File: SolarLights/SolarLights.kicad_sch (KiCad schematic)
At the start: 25 parts, among them J1 BAT GND, J2 BAT 12V, J3 SWITCH IN, J4 SWITCH 12V, J5 SWITCH GND, J6 PROG, U1 ATtiny1616

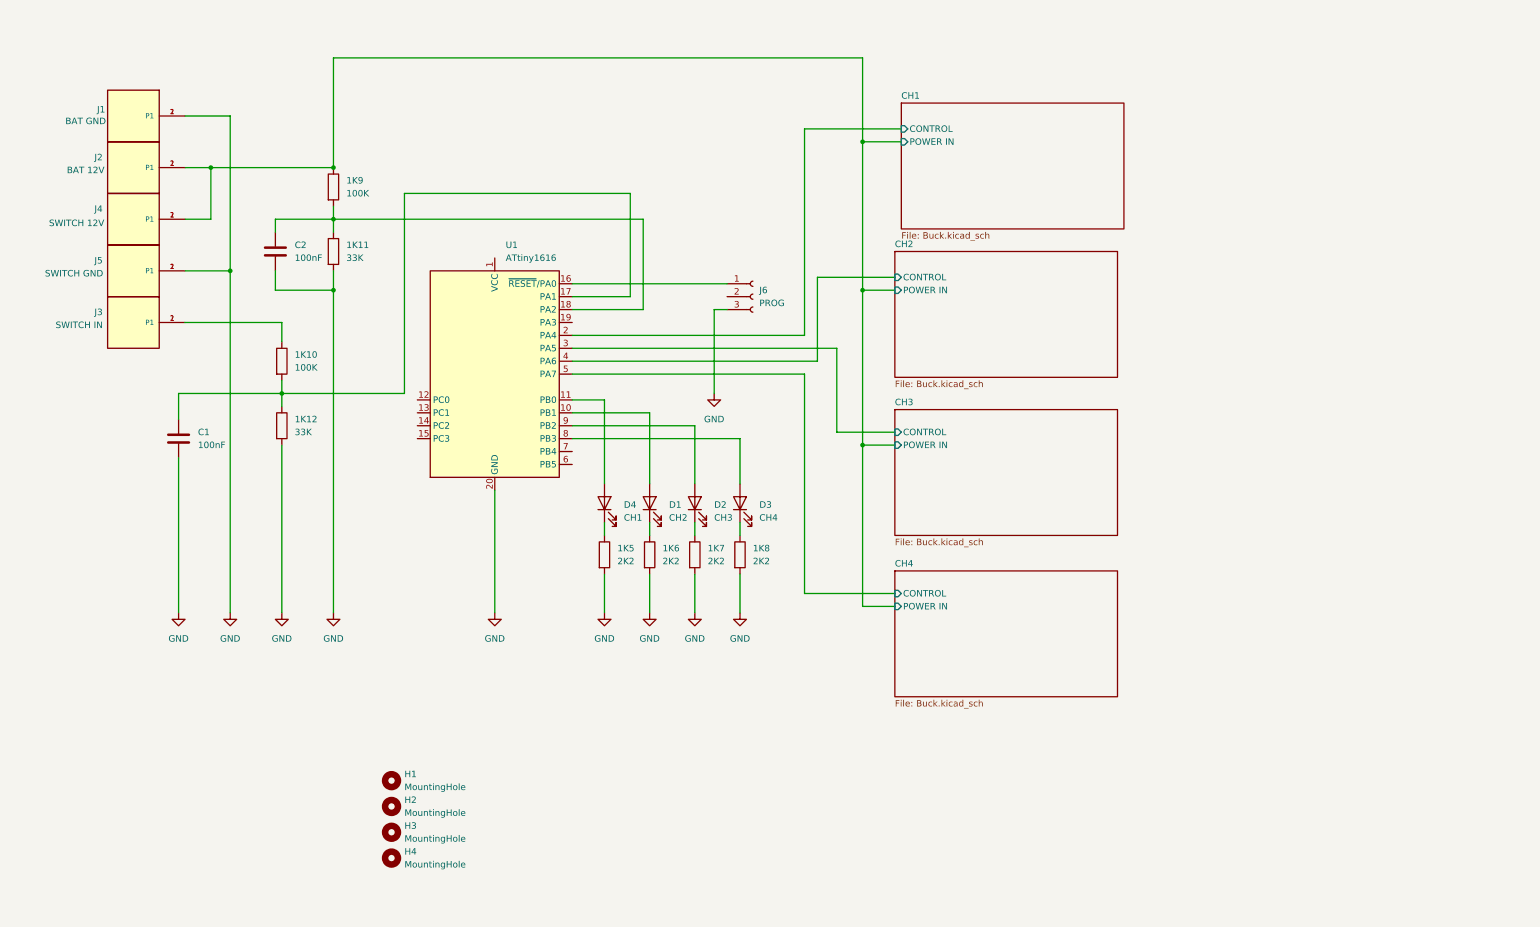
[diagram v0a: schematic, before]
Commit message: solar lights
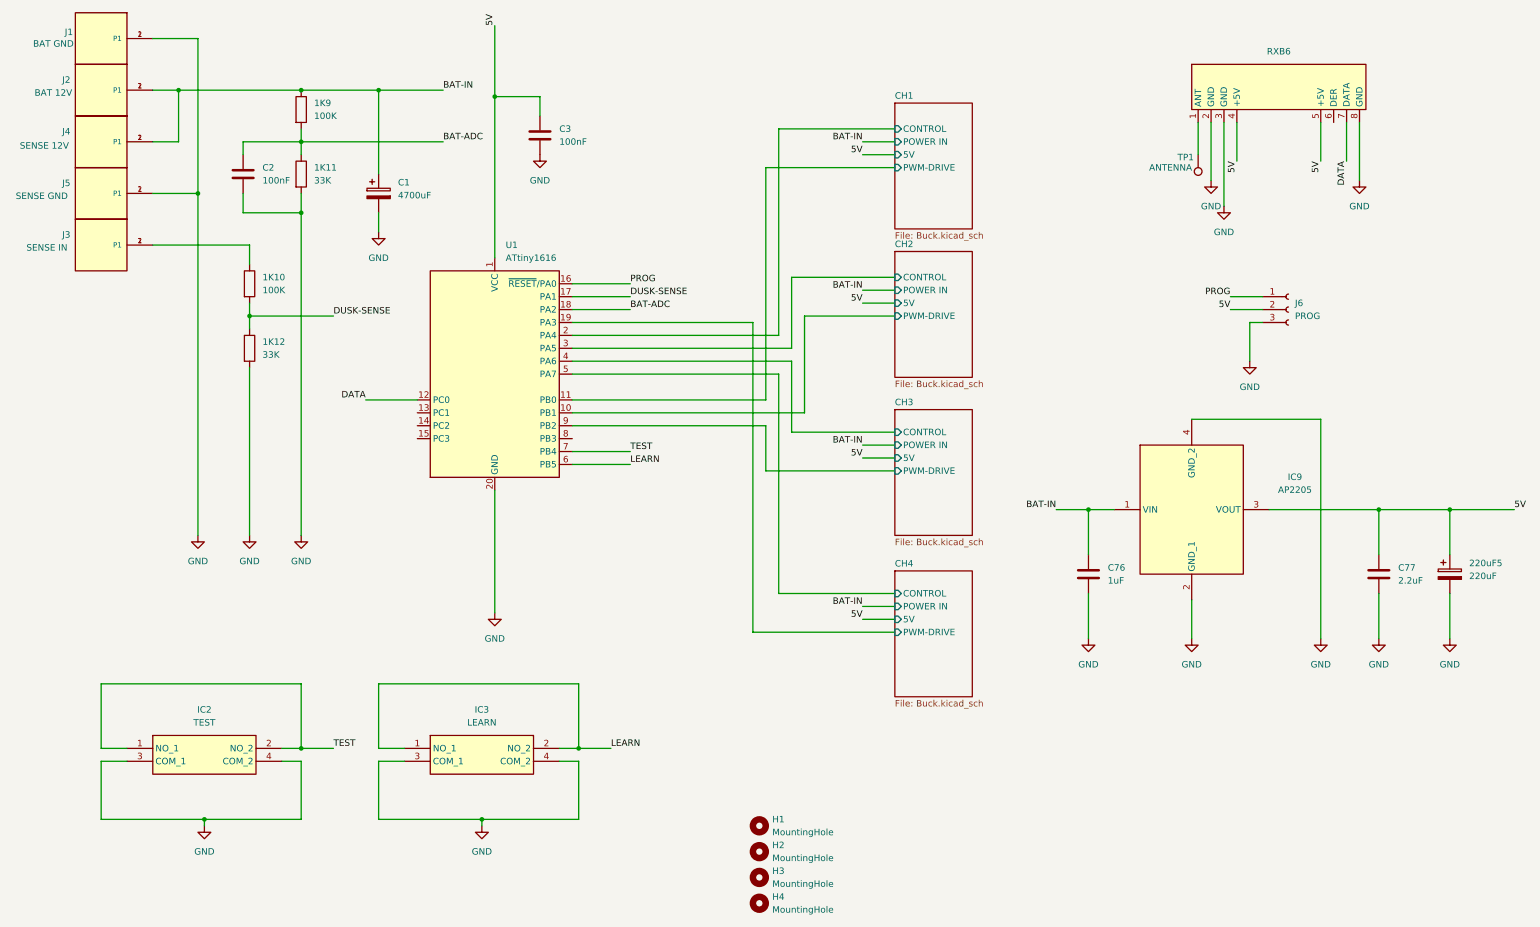
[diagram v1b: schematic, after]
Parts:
- removed 1K5, 1K6, 1K7, 1K8: 2K2, Resistor_SMD:R_0805_2012Metric_Pad1.20x1.40mm_HandSolder, symbol Device:R
- removed C1: 100nF, Capacitor_SMD:C_1206_3216Metric_Pad1.33x1.80mm_HandSolder, symbol Device:C
- removed D1: CH2, LED_THT:LED_D5.0mm, symbol Device:LED
- removed D2: CH3, LED_THT:LED_D5.0mm, symbol Device:LED
- removed D3: CH4, LED_THT:LED_D5.0mm, symbol Device:LED
- removed D4: CH1, LED_THT:LED_D5.0mm, symbol Device:LED
- added 220uF5: 220uF, Capacitor_THT:CP_Radial_D6.3mm_P2.50mm, symbol Device:C_Polarized
- added C1: 4700uF, Capacitor_THT:CP_Radial_D16.0mm_P7.50mm, symbol Device:C_Polarized
- added C3: 100nF, Capacitor_SMD:C_1206_3216Metric_Pad1.33x1.80mm_HandSolder, symbol Device:C
- added C76: 1uF, Capacitor_SMD:C_1206_3216Metric_Pad1.33x1.80mm_HandSolder, symbol Device:C
- added C77: 2.2uF, Capacitor_SMD:C_0805_2012Metric_Pad1.18x1.45mm_HandSolder, symbol Device:C
- added IC2: TEST, Custom:TS026650BK100SCRD, symbol Custom:TS02-66-50-BK-100-SCR-D
- added IC3: LEARN, Custom:TS026650BK100SCRD, symbol Custom:TS02-66-50-BK-100-SCR-D
- added IC9: AP2205, Custom:2205, symbol Custom:AP2205-50YR-13
- added RXB6: (no value), Custom:RXB6, symbol Custom:RXB6
- added TP1: ANTENNA, TestPoint:TestPoint_Pad_D4.0mm, symbol Connector:TestPoint
- J3: value SWITCH IN -> SENSE IN
- J4: value SWITCH 12V -> SENSE 12V
- J5: value SWITCH GND -> SENSE GND
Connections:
- net CH2/CONTROL: now also U1.3 (PA5); no longer U1.4 (PA6)
- net CH3/CONTROL: now also U1.4 (PA6); no longer U1.3 (PA5)
- net GND: now also 220uF5.2, C1.2, C3.2, C76.1, C77.2, IC2.3 (COM_1), IC2.4 (COM_2), IC3.3 (COM_1), IC3.4 (COM_2), IC9.2 (GND_1), IC9.4 (GND_2), RXB6.2 (GND), RXB6.3 (GND), RXB6.8 (GND)
- net BAT-ADC: now reaches 1K11.1, 1K9.2, C2.1, U1.18 (PA2)
- net CH3/PWM-DRIVE: now reaches U1.9 (PB2)
- net DUSK-SENSE: now reaches 1K10.2, 1K12.1, U1.17 (PA1)
- net CH2/PWM-DRIVE: now reaches U1.10 (PB1)
- net CH1/PWM-DRIVE: now reaches U1.11 (PB0)
- net 5V: now reaches U1.1 (VCC)
- net 5V: now also J6.2 (Pin_2), 220uF5.1, C3.1, C77.1, IC9.3 (VOUT), RXB6.4 (+5V), RXB6.5 (+5V)
- net DATA: now reaches U1.12 (PC0)
- net DATA: now also RXB6.7 (DATA)
- net PROG: now reaches J6.1 (Pin_1), U1.16 (~{RESET}/PA0)
- net CH4/PWM-DRIVE: now reaches U1.19 (PA3)
- net LEARN: now reaches U1.6 (PB5)
- net LEARN: now also IC3.1 (NO_1), IC3.2 (NO_2)
- net TEST: now reaches U1.7 (PB4)
- net TEST: now also IC2.1 (NO_1), IC2.2 (NO_2)
- net CH1/POWER IN renamed BAT-IN
- net BAT-IN: now also C1.1, C76.2, IC9.1 (VIN)
- new net: RXB6.1 (ANT), TP1.1
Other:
- sheet CH1 ports: added 5V, PWM-DRIVE; removed none
- sheet CH2 ports: added 5V, PWM-DRIVE; removed none
- sheet CH3 ports: added 5V, PWM-DRIVE; removed none
- sheet CH4 ports: added 5V, PWM-DRIVE; removed none
- moved on the sheet: 1K10, 1K11, 1K12, 1K9, C2, H1, H2, H3, H4, J1, J2, J3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
